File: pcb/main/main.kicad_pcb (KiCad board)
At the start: 2 copper layers, 172.1 x 109.2 mm, 74 parts, among them J1 Conn_01x04, J10 JTAG, J2 USB_B, J3 Trackball_conn, J4 ROW0, J5 RJ45, J6 ROW1, J7 ROW2, J8 ROW3, J9 STLink, SW1 SW40, SW2 SW41, SW3 SW42, SW4 SW43, SW5 RST_SW, SW6 BOOT0, SW7 BOOT1, U1 3.3v regul, U2 STM32F103C8Tx, Y1 32.768kHz, Y2 8MHz

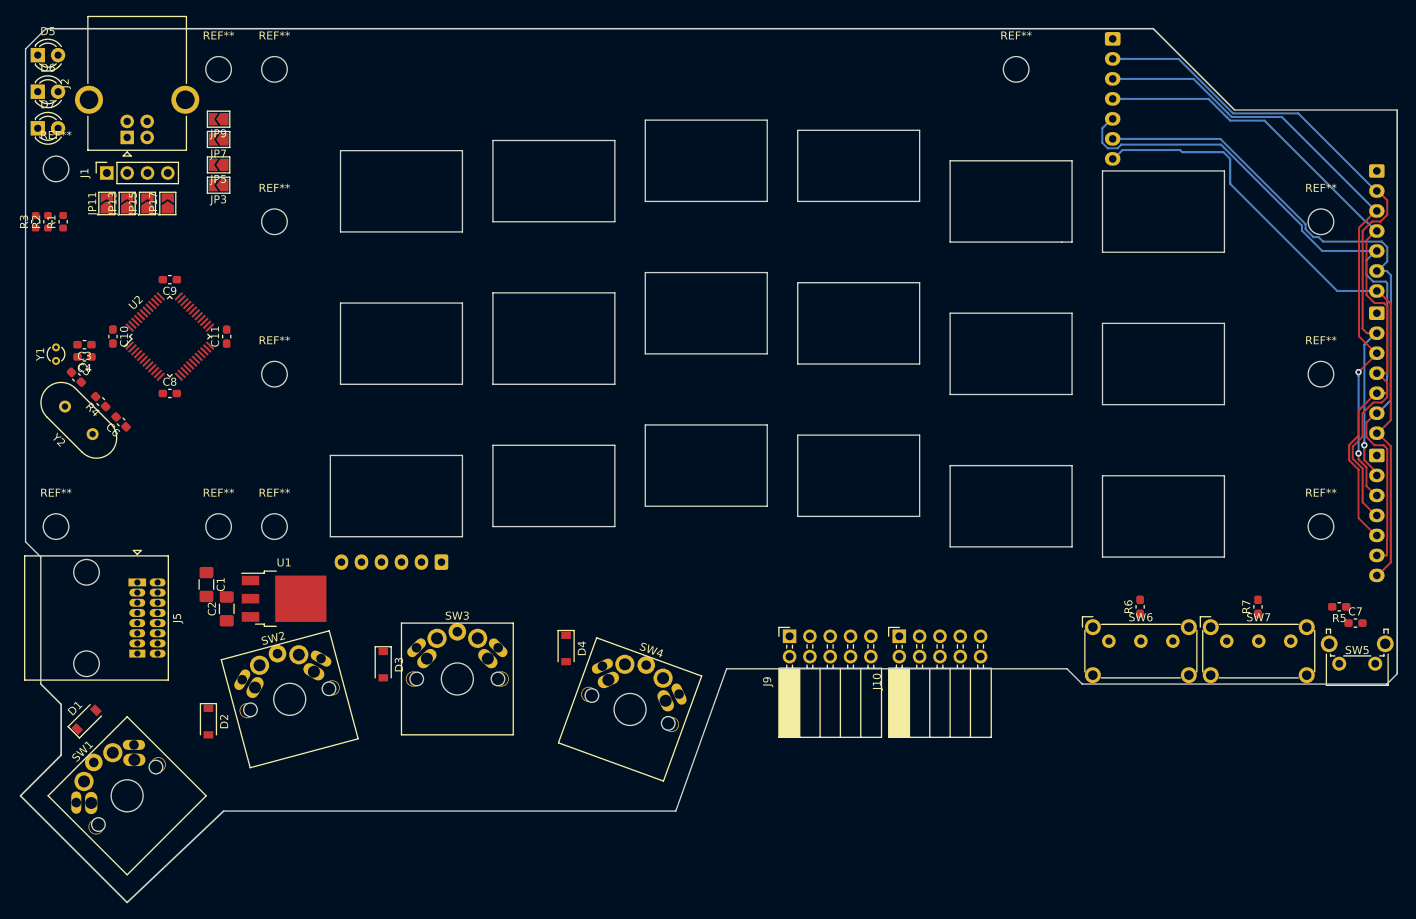
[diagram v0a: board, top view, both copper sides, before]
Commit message: keyboard pcb
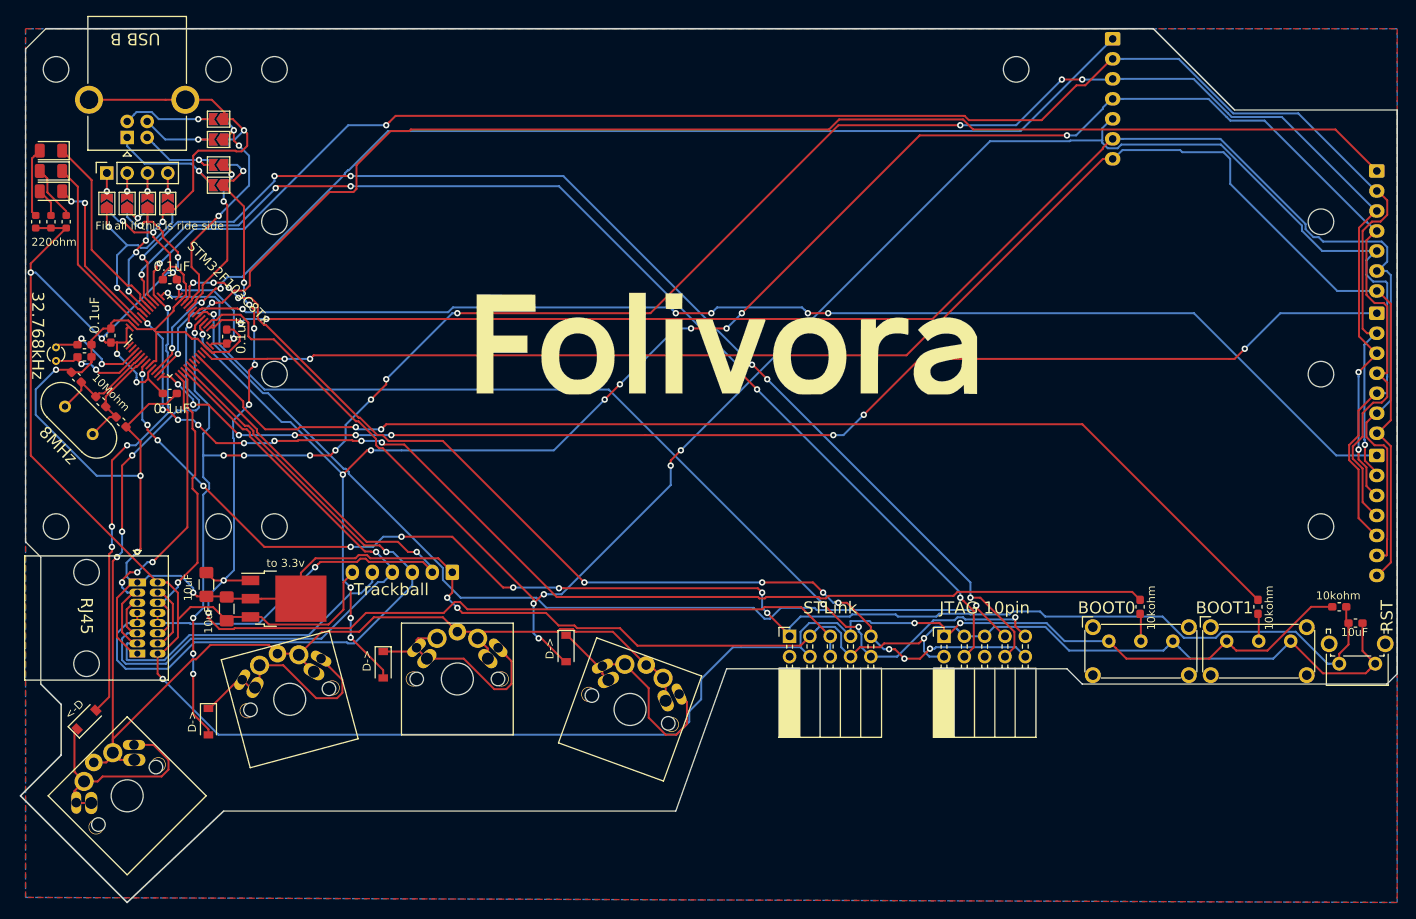
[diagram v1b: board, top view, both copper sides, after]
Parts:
- added G***: LOGO, folivora:logo, B.Cu at (189.2, 124.5)
- added G***: LOGO, folivora:logo, F.Cu at (172.7, 78.7)
- added G***: LOGO, folivora:logo, F.Cu at (189.2, 61.0)
- added G***: LOGO, folivora:logo, F.Cu at (189.2, 124.5)
- D5, D6, D7: footprint LED_THT:LED_D3.0mm -> LED_SMD:LED_1206_3216Metric
- moved D5 17.1 mm to (104.8, 105.4), turned to 180 degrees
- moved REF** 12.4 mm to (105.4, 90.2)
- moved D6 10.0 mm to (104.8, 102.9), turned to 180 degrees
- moved J10 5.59 mm to (216.4, 161.0)
- moved D7 3.25 mm to (104.8, 100.3), turned to 180 degrees
- moved R2 2.29 mm to (106.7, 109.2)
- moved J3 1.85 mm to (154.9, 153.0)
- moved R1 1.52 mm to (104.8, 109.2)
- moved C10 0.28 mm to (112.3, 123.4), turned to 90 degrees
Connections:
- J3 pad 1: +3V3 -> GND
- J3 pad 2: /SS_T -> /MOSI
- J3 pad 3: /SCK -> /MISO
- J3 pad 4: /MISO -> /SCK
- J3 pad 5: /MOSI -> /SS_T
- J3 pad 6: GND -> +3V3
- JP12 pad 1: +5V -> +3V3
- JP15 pad 1: +5V -> +3V3
- U2 pad 21: /LED3 -> Net-(U2-Pad21)
- U2 pad 22: /D- -> /READ5
- U2 pad 25: /D+ -> /READ4
- U2 pad 32: /READ5 -> /D-
- U2 pad 33: /READ4 -> /D+
- U2 pad 41: Net-(U2-Pad41) -> /LED3
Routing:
- net GND: track 0.00 -> 364.3 mm, vias 0 -> 11
- net +3V3: track 0.00 -> 345.9 mm, vias 0 -> 12
- net /READ0: track 80.8 -> 272.5 mm, vias 1 -> 7
- net /READ1: track 79.4 -> 269.4 mm, vias 2 -> 16
- net /RST: track 0.00 -> 184.1 mm, vias 0 -> 10
- net /SELECT1: track 0.00 -> 172.8 mm, vias 0 -> 2
- net /READ2: track 83.4 -> 254.0 mm, vias 0 -> 12
- net /READ3: track 86.7 -> 250.9 mm, vias 0 -> 5
- net /SELECT2: track 0.00 -> 161.7 mm, vias 0 -> 9
- net /SELECT4: track 0.00 -> 159.2 mm, vias 0 -> 4
- net /SELECT3: track 0.00 -> 156.6 mm, vias 0 -> 5
- net +5V: track 0.00 -> 154.1 mm, vias 0 -> 8
- net /JTDO: track 0.00 -> 148.1 mm, vias 0 -> 6
- net /BOOT1: track 0.00 -> 146.2 mm, vias 0 -> 2
- net /BOOT0: track 0.00 -> 146.0 mm, vias 0 -> 8
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- added copper zone on B.Cu, net GND
- added copper zone on F.Cu, net GND
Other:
- outline, holes or cut-outs redrawn
- rule trace_min: 0.2 -> 0
- board text added: "0.1uF"
- board text added: "10Mohm"
- board text added: "10kohm"
- board text added: "10uF"
- board text added: "220ohm"
- board text added: "32.768kHz"
- board text added: "8MHz"
- board text added: "<-D"
- board text added: "BOOT0"
- board text added: "BOOT1"
- board text added: "D->"
- board text added: "Fill all if this is ride side"
- board text added: "JTAG 10pin"
- board text added: "RJ45"
- board text added: "RST"
- board text added: "STLink"
- board text added: "STM32F103C8Tx"
- board text added: "Trackball"
- board text added: "USB B"
- board text added: "to 3.3v"

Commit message: fix design
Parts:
- removed the REF** at (263.5, 147.3)
- removed the REF** at (263.5, 128.3)
- removed the REF** at (125.7, 90.2)
- added REF**: MountingHole_2.2mm_M2, MountingHole:MountingHole_2.2mm_M2, F.Cu at (55.9, 72.4)
- added REF**: MountingHole_2.2mm_M2, MountingHole:MountingHole_2.2mm_M2, F.Cu at (74.9, 59.7)
- added REF**: MountingHole_2.2mm_M2, MountingHole:MountingHole_2.2mm_M2, F.Cu at (113.0, 59.7)
- added REF**: MountingHole_2.2mm_M2, MountingHole:MountingHole_2.2mm_M2, F.Cu at (113.0, 72.4)
- added REF**: MountingHole_2.2mm_M2, MountingHole:MountingHole_2.2mm_M2, F.Cu at (55.9, 53.3)
- added REF**: MountingHole_2.2mm_M2, MountingHole:MountingHole_2.2mm_M2, F.Cu at (132.1, 40.6)
- added REF**: MountingHole_2.2mm_M2, MountingHole:MountingHole_2.2mm_M2, F.Cu at (94.0, 53.3)
- added REF**: MountingHole_2.2mm_M2, MountingHole:MountingHole_2.2mm_M2, F.Cu at (94.0, 40.6)
- added REF**: MountingHole_2.2mm_M2, MountingHole:MountingHole_2.2mm_M2, F.Cu at (151.1, 53.3)
- added REF**: MountingHole_2.2mm_M2, MountingHole:MountingHole_2.2mm_M2, F.Cu at (55.9, 40.6)
- added REF**: MountingHole_2.2mm_M2, MountingHole:MountingHole_2.2mm_M2, F.Cu at (151.1, 40.6)
- added REF**: MountingHole_2.2mm_M2, MountingHole:MountingHole_2.2mm_M2, F.Cu at (132.1, 59.7)
- added REF**: MountingHole_2.2mm_M2, MountingHole:MountingHole_2.2mm_M2, F.Cu at (132.1, 53.3)
- added REF**: MountingHole_2.2mm_M2, MountingHole:MountingHole_2.2mm_M2, F.Cu at (74.9, 53.3)
- added REF**: MountingHole_2.2mm_M2, MountingHole:MountingHole_2.2mm_M2, F.Cu at (74.9, 40.6)
- added REF**: MountingHole_2.2mm_M2, MountingHole:MountingHole_2.2mm_M2, F.Cu at (113.0, 40.6)
- added REF**: MountingHole_2.2mm_M2, MountingHole:MountingHole_2.2mm_M2, F.Cu at (113.0, 53.3)
- added REF**: MountingHole_2.2mm_M2, MountingHole:MountingHole_2.2mm_M2, F.Cu at (55.9, 34.3)
- added REF**: MountingHole_2.2mm_M2, MountingHole:MountingHole_2.2mm_M2, F.Cu at (132.1, 21.6)
- added REF**: MountingHole_2.2mm_M2, MountingHole:MountingHole_2.2mm_M2, F.Cu at (94.0, 34.3)
- added REF**: MountingHole_2.2mm_M2, MountingHole:MountingHole_2.2mm_M2, F.Cu at (94.0, 21.6)
- added REF**: MountingHole_2.2mm_M2, MountingHole:MountingHole_2.2mm_M2, F.Cu at (151.1, 34.3)
- added REF**: MountingHole_2.2mm_M2, MountingHole:MountingHole_2.2mm_M2, F.Cu at (94.0, 72.4)
- added REF**: MountingHole_2.2mm_M2, MountingHole:MountingHole_2.2mm_M2, F.Cu at (55.9, 21.6)
- added REF**: MountingHole_2.2mm_M2, MountingHole:MountingHole_2.2mm_M2, F.Cu at (151.1, 21.6)
- added REF**: MountingHole_2.2mm_M2, MountingHole:MountingHole_2.2mm_M2, F.Cu at (132.1, 34.3)
- added REF**: MountingHole_2.2mm_M2, MountingHole:MountingHole_2.2mm_M2, F.Cu at (74.9, 34.3)
- added REF**: MountingHole_2.2mm_M2, MountingHole:MountingHole_2.2mm_M2, F.Cu at (74.9, 21.6)
- added REF**: MountingHole_2.2mm_M2, MountingHole:MountingHole_2.2mm_M2, F.Cu at (113.0, 21.6)
- added REF**: MountingHole_2.2mm_M2, MountingHole:MountingHole_2.2mm_M2, F.Cu at (113.0, 34.3)
- added REF**: MountingHole_2.2mm_M2, MountingHole:MountingHole_2.2mm_M2, F.Cu at (94.0, 59.7)
- added REF**: MountingHole_3.2mm_M3, MountingHole:MountingHole_3.2mm_M3, F.Cu at (161.9, 66.0)
- added REF**: MountingHole_3.2mm_M3, MountingHole:MountingHole_3.2mm_M3, F.Cu at (161.9, 47.0)
- added REF**: MountingHole_3.2mm_M3, MountingHole:MountingHole_3.2mm_M3, F.Cu at (24.1, 5.08)
- added REF**: MountingHole_2.2mm_M2, MountingHole:MountingHole_2.2mm_M2, F.Cu at (55.9, 15.2)
- added REF**: MountingHole_2.2mm_M2, MountingHole:MountingHole_2.2mm_M2, F.Cu at (151.1, 72.4)
- added REF**: MountingHole_2.2mm_M2, MountingHole:MountingHole_2.2mm_M2, F.Cu at (55.9, 2.54)
- added REF**: MountingHole_2.2mm_M2, MountingHole:MountingHole_2.2mm_M2, F.Cu at (74.9, 2.54)
- added REF**: MountingHole_2.2mm_M2, MountingHole:MountingHole_2.2mm_M2, F.Cu at (74.9, 15.2)
- added REF**: MountingHole_2.2mm_M2, MountingHole:MountingHole_2.2mm_M2, F.Cu at (94.0, 2.54)
- added REF**: MountingHole_2.2mm_M2, MountingHole:MountingHole_2.2mm_M2, F.Cu at (94.0, 15.2)
- added REF**: MountingHole_2.2mm_M2, MountingHole:MountingHole_2.2mm_M2, F.Cu at (113.0, 2.54)
- added REF**: MountingHole_2.2mm_M2, MountingHole:MountingHole_2.2mm_M2, F.Cu at (113.0, 15.2)
- added REF**: MountingHole_2.2mm_M2, MountingHole:MountingHole_2.2mm_M2, F.Cu at (55.9, 59.7)
- added REF**: MountingHole_2.2mm_M2, MountingHole:MountingHole_2.2mm_M2, F.Cu at (151.1, 59.7)
- added REF**: MountingHole_2.2mm_M2, MountingHole:MountingHole_2.2mm_M2, F.Cu at (132.1, 72.4)
- added REF**: MountingHole_2.2mm_M2, MountingHole:MountingHole_2.2mm_M2, F.Cu at (74.9, 72.4)
- J4, J6, J7, J8: footprint Connector_JST:JST_XH_S07B-XH-A_1x07_P2.50mm_Horizontal -> Connector_PinSocket_2.00mm:PinSocket_1x07_P2.00mm_Vertical; moved to F.Cu
- SW6, SW7: footprint Button_Switch_THT:SW_E-Switch_EG1224_SPDT_Angled -> Button_Switch_THT:SW_CuK_OS102011MA1QN1_SPDT_Angled
- moved J3 155.8 mm to (21.6, 72.4), turned to 270 degrees
- moved U1 150.0 mm to (19.7, 59.1), turned to 45 degrees
- moved C2 145.1 mm to (15.2, 64.8), turned to 135 degrees
- moved C1 144.7 mm to (10.8, 64.8), turned to 315 degrees
- moved J4 134.3 mm to (132.1, 3.17), turned to 0 degrees
- moved REF** 132.5 mm to (3.81, 5.08)
- moved J2 131.0 mm to (12.7, 16.0)
- moved J6 130.6 mm to (168.3, 21.6), turned to 0 degrees
- moved C5 130.1 mm to (6.35, 47.4)
- moved D5 130.1 mm to (3.17, 24.1)
- moved D6 130.1 mm to (3.17, 21.6)
- moved D7 130.1 mm to (3.17, 19.1)
- moved J1 130.1 mm to (10.2, 21.8)
- moved J9 130.1 mm to (95.5, 79.8)
- moved JP10 130.1 mm to (10.2, 25.7)
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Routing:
- net +3V3: track 345.9 -> 289.7 mm, vias 12 -> 16
- net /MOSI: track 81.3 -> 42.6 mm, vias 2 -> 0
- net /READ5: track 205.5 -> 243.8 mm, vias 2 -> 1
- net /MISO: track 90.1 -> 55.2 mm
- net /READ1: track 269.4 -> 299.2 mm, vias 16 -> 5
- net /READ4: track 208.3 -> 232.3 mm, vias 2 -> 4
- net /READ2: track 254.0 -> 276.7 mm, vias 12 -> 6
- net /SCK: track 86.1 -> 63.6 mm, vias 1 -> 2
- net /SWCLK: track 135.4 -> 155.7 mm, vias 4 -> 1
- net /SS_T: track 81.1 -> 64.3 mm, vias 3 -> 2
- net /JNTRST: track 142.2 -> 126.0 mm, vias 6 -> 1
- net /JTDO: track 148.1 -> 132.9 mm, vias 6 -> 1
- net GND: track 364.3 -> 350.5 mm, vias 11 -> 13
- net /READ3: track 250.9 -> 262.7 mm, vias 5 -> 8
- net /SELECT1: track 172.8 -> 163.0 mm, vias 2 -> 1
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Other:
- board size 172.1 x 109.2 mm -> 172.1 x 113 mm
- net class Default: clearance 0.2 -> 0.16; trace_width 0.25 -> 0.2; via_dia 0.8 -> 0.5; via_drill 0.4 -> 0.3
- rule trace_clearance: 0.2 -> 0.16
